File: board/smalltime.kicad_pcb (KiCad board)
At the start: 2 copper layers, 80 x 56 mm, 45 parts, among them IC1 STM32F030K6T6, IC2 DS3231MZ, IC3 ADP3338, J1 MICROUSB, P1 SWD, P2 SWD_TC, Q1 TEPT4400, Q2 Q_NMOS_GDS, Q3 Q_NMOS_GDS, Q4 Q_NMOS_GDS, Q5 Q_NMOS_GDS, Q6 Q_NMOS_GDS, Q7 Q_NMOS_GDS, Q8 Q_NMOS_GDS, Q9 Q_NMOS_GDS, SW1 INC, SW2 SET, U1 DIG1, U2 DIG2, U3 DIG3, U4 DIG4, U5 DIG5, U6 DIG6, U7 DIG7, U8 DIG8

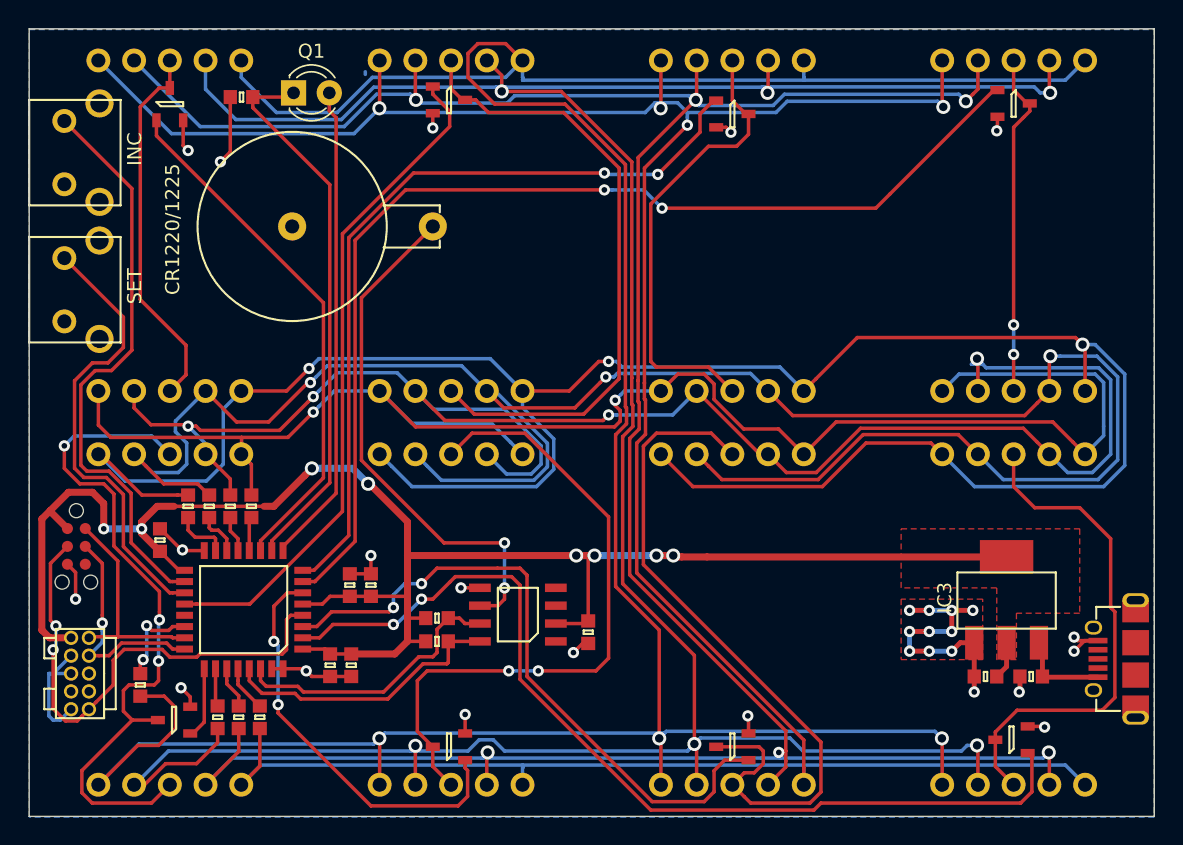
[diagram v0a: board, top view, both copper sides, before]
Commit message: Schematic checking/finishing
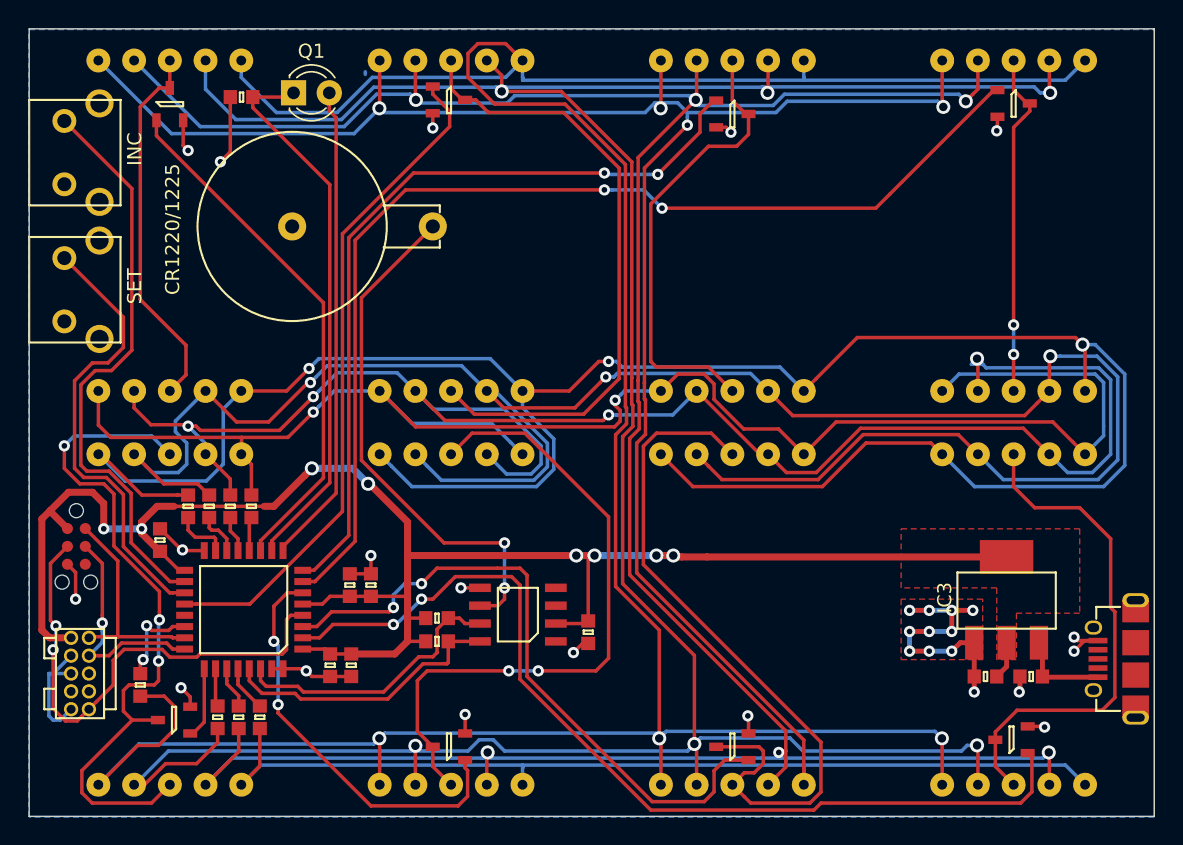
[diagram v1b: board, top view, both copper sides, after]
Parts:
- Q2, Q3, Q4, Q5, Q6, Q7, Q8, Q9: value Q_NMOS_GDS -> Q_NMOS_GSD
- R10, R11, R4, R5, R6, R7, R8, R9: value 300 -> 160
